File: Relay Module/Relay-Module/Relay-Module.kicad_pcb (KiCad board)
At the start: 2 copper layers, 207.3 x 99.3 mm, 48 parts, among them J1 0039301039, J10 0039301039, J11 0039281023, J12 0039281023, J13 0039281023, J14 0039281023, J15 0039281023, J16 0039281023, J17 0039301039, J18 0039301039, J19 0039281023, J2 0039301039, J20 0039281023, J21 0039281023, J22 0039281023, J23 0039281023, J24 0039281023, J25 0039301039, J26 0039301039, J27 0039281023, J28 0039281023, J29 0039281023, J3 0039281023, J30 0039281023, J31 0039281023, J32 0039281023, J4 0039281023, J5 0039281023, J6 0039281023, J7 0039281023, J8 0039281023, J9 0039301039, K1 T77S1D3-05, K2 T77S1D3-05, K3 T77S1D3-05, K4 T77S1D3-05, K5 T77S1D3-05, K6 T77S1D3-05, K7 T77S1D3-05, K8 T77S1D3-05

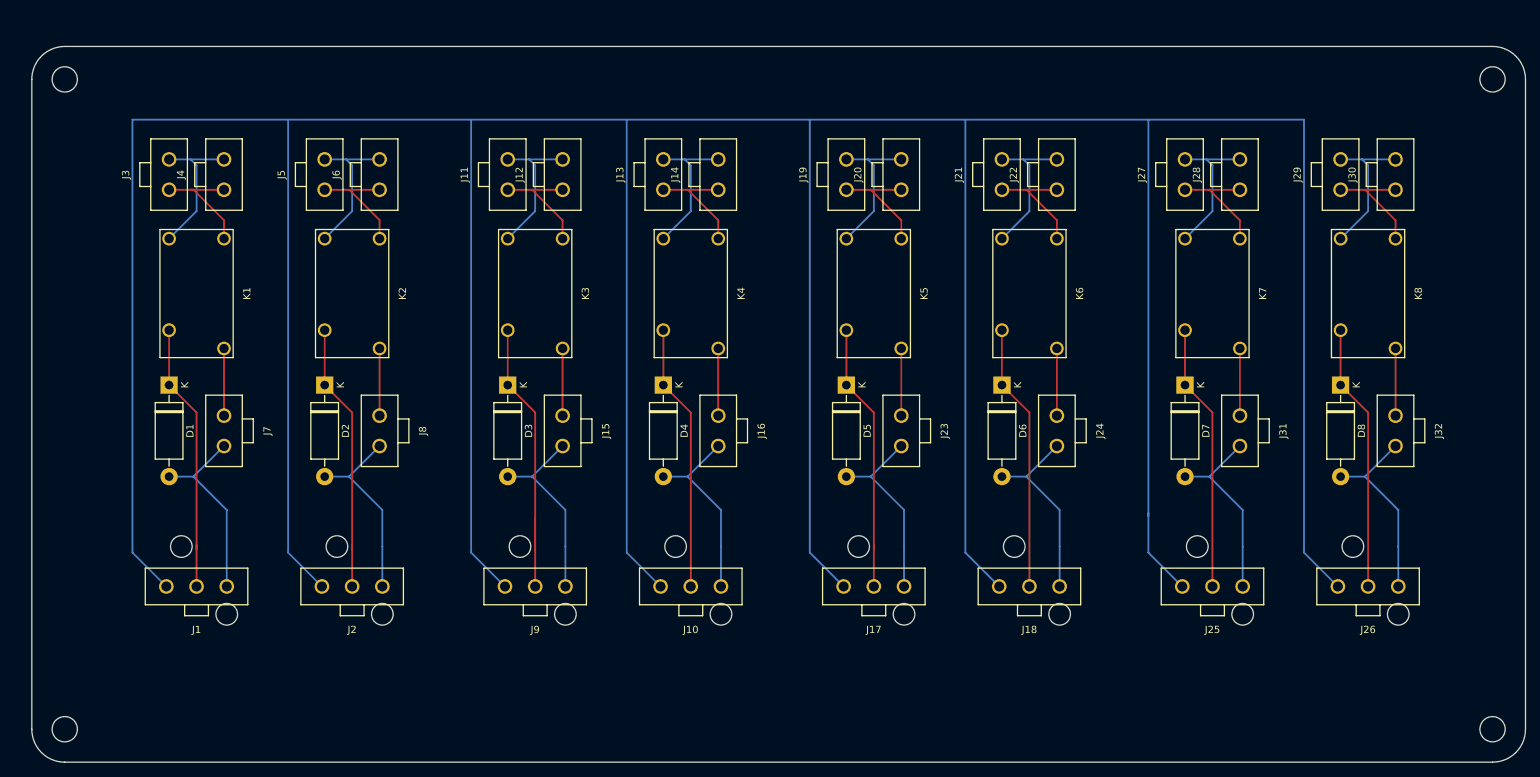
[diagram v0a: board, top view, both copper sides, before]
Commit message: Relay module update and trigger module creation
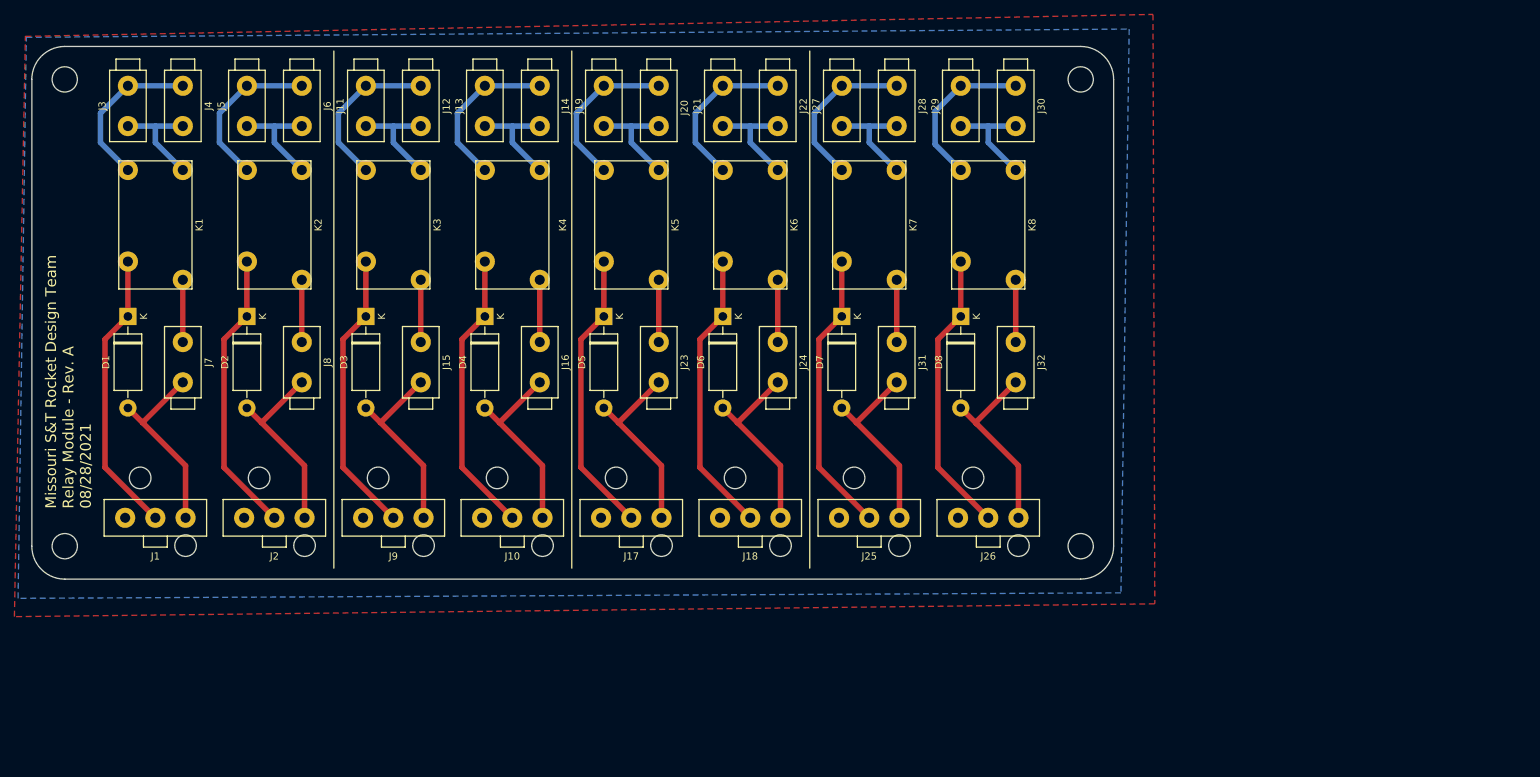
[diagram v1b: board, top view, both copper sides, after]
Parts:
- moved D8 53.6 mm to (167.0, 75.6)
- moved J26 53.6 mm to (170.8, 103.5)
- moved J29 53.6 mm to (167.0, 46.4)
- moved J30 53.6 mm to (174.6, 46.4)
- moved J32 53.6 mm to (174.6, 81.9)
- moved K8 53.6 mm to (170.8, 62.9)
- moved D7 48.6 mm to (150.5, 75.6)
- moved J25 48.6 mm to (154.3, 103.5)
- moved J27 48.6 mm to (150.5, 46.4)
- moved J28 48.6 mm to (158.1, 46.4)
- moved J31 48.6 mm to (158.1, 81.9)
- moved K7 48.6 mm to (154.3, 62.9)
- moved J18 39.9 mm to (137.8, 103.5)
- moved J22 39.9 mm to (141.6, 46.4)
- moved J24 39.9 mm to (141.6, 81.9)
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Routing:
- net GND: track 696.7 -> 0.00 mm
- net Net-(D7-Pad1): track 37.1 -> 40.1 mm
- net Net-(D4-Pad1): track 37.1 -> 39.8 mm
- net Net-(D6-Pad1): track 37.1 -> 39.8 mm
- net Net-(D8-Pad1): track 37.1 -> 39.8 mm
- net Net-(D5-Pad1): track 37.8 -> 39.8 mm
- net Net-(D2-Pad1): track 37.8 -> 39.8 mm
- net Net-(D1-Pad1): track 37.8 -> 39.8 mm
- net Net-(J13-Pad2): track 20.5 -> 22.5 mm
- net Net-(J3-Pad2): track 20.5 -> 22.5 mm
- net Net-(J27-Pad2): track 20.5 -> 22.5 mm
- net Net-(J11-Pad2): track 20.5 -> 22.5 mm
- net Net-(J19-Pad2): track 20.5 -> 22.5 mm
- net Net-(J5-Pad2): track 20.5 -> 22.5 mm
- net Net-(J21-Pad2): track 20.5 -> 22.5 mm
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- added copper zone on B.Cu, net GND
- added copper zone on F.Cu, net GND
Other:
- board size 207.3 x 99.3 mm -> 150.1 x 73.9 mm
- board text added: "Missouri S&T Rocket Design Team Relay Module - Rev. A 08/28/2021"
